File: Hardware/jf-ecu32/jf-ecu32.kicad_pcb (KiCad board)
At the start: 2 copper layers, 71.2 x 47 mm, 84 parts, among them J1 GAZ, J10 k, J11 RPM, J12 S.PORT, J13 PPM/PWM, J14 PUMP1, J15 PUMP1, J16 PPM/PWM, J17 PUMP2, J18 PUMP2, J19 UART0, J2 AUX, J3 PPM/PWM, J4 STARTER, J5 GLOW, J6 VANNE KEROSTART, J7 VANNE KERO, J8 BATTERY 2S/3S, J9 STARTER, Q1 AO3400A, Q2 QM6006D, Q3 AO3400A, Q4 QM6006D, Q5 QM6006D, Q6 QM6006D, Q7 AO3401A, U1 ESP32-WROOM-32D, U2 4050, U3 MAX31855KASA, U4 AMS1117-3.3, U5 4050, U6 AMS1117-5.0, U7 OPA340NA, U8 LM4040DBZ-2.5

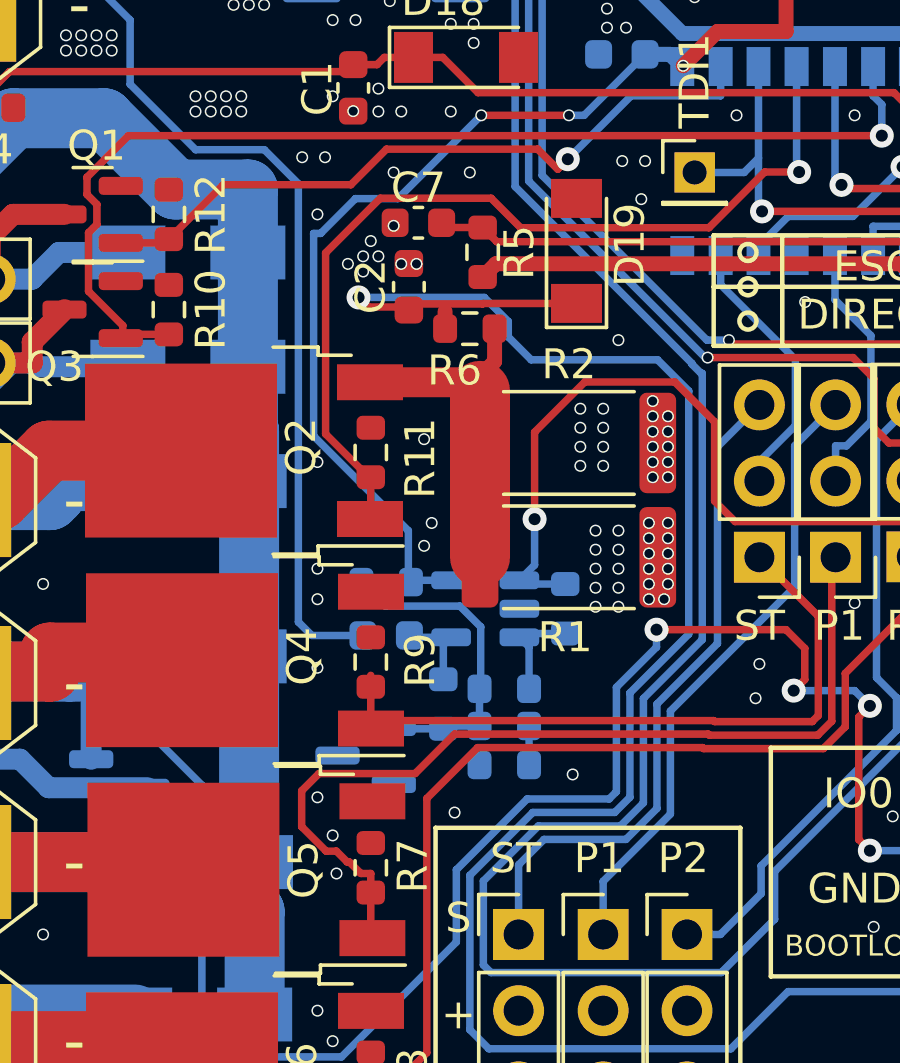
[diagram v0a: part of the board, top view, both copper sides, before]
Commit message: RPM problem
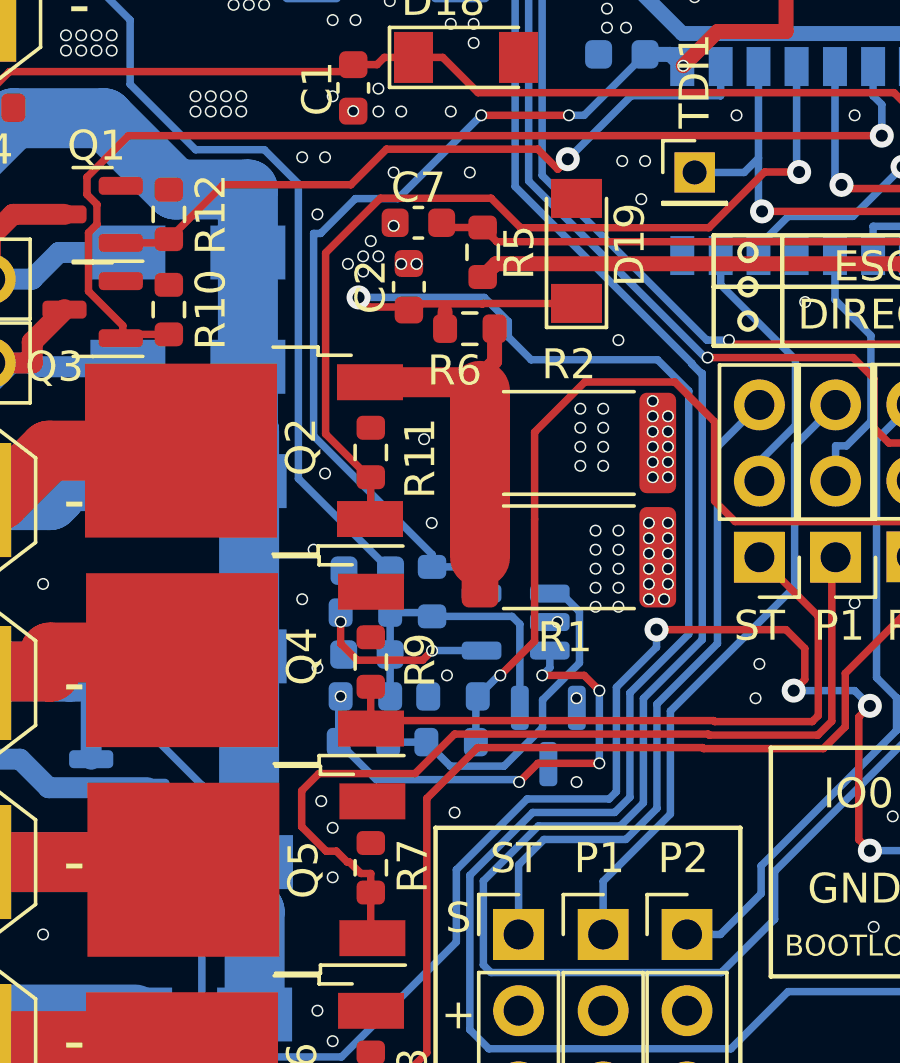
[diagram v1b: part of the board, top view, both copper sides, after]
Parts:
- added C12: 0.1µF, Capacitor_SMD:C_0603_1608Metric, B.Cu at (36.4, 179.1)
- R18: value 100 -> 20K
- R19: value 7K -> 20K
- R21: value 510K -> 20K
- moved R21 8.06 mm to (36.3, 182.1), turned to 0 degrees
- moved U8 6.12 mm to (42.5, 181.9), turned to -90 degrees
- moved R20 4.64 mm to (36.4, 180.5), turned to 180 degrees
- moved R17 4.00 mm to (36.4, 177.7), turned to 180 degrees
- moved C4 2.25 mm to (36.5, 176.3), turned to 180 degrees
- moved R19 1.97 mm to (39.3, 180.5), turned to 0 degrees
- moved R18 1.93 mm to (39.3, 182.1), turned to 180 degrees
- moved R22 1.56 mm to (38.6, 177.0), turned to -90 degrees
- moved U7 1.11 mm to (41.4, 178.1)
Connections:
- R18 pad 1: GND -> RPM-2
- R18 pad 2: Net-(R18-Pad2) -> Net-(R21-Pad2)
- R19 pad 1: Net-(R18-Pad2) -> GND
- R19 pad 2: +2V5 -> RPM-2
- R21 pad 2: RPM-2 -> Net-(R21-Pad2)
- U7 pad 1: RPM-2 -> Net-(R21-Pad2)
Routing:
- net Net-(R20-Pad2): track 3.43 -> 16.5 mm, vias 0 -> 5
- net Net-(R21-Pad2): track 0.00 -> 11.6 mm
- net Net-(C4-Pad2): track 2.92 -> 7.72 mm, vias 0 -> 2
- net RPM-2: track 36.5 -> 40.9 mm
- net RPM: track 34.0 -> 31.2 mm
- net Net-(R18-Pad2): track 1.30 -> 0.00 mm
- net +2V5: track 10.8 -> 10.1 mm
- net GND: vias 361 -> 363
